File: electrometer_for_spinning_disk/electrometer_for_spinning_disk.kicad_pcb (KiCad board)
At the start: 2 copper layers, 40 x 60 mm, 22 parts, among them J1 Conn_01x01_Pin, J2 Conn_01x03_Pin, J3 Screw_Terminal_01x03, J4 PRT-14417, J5 Conn_01x01_Pin, J7 Conn_01x03_Pin, U1 LMC6082, U2 ADS1115IDGS, U3 REF3025

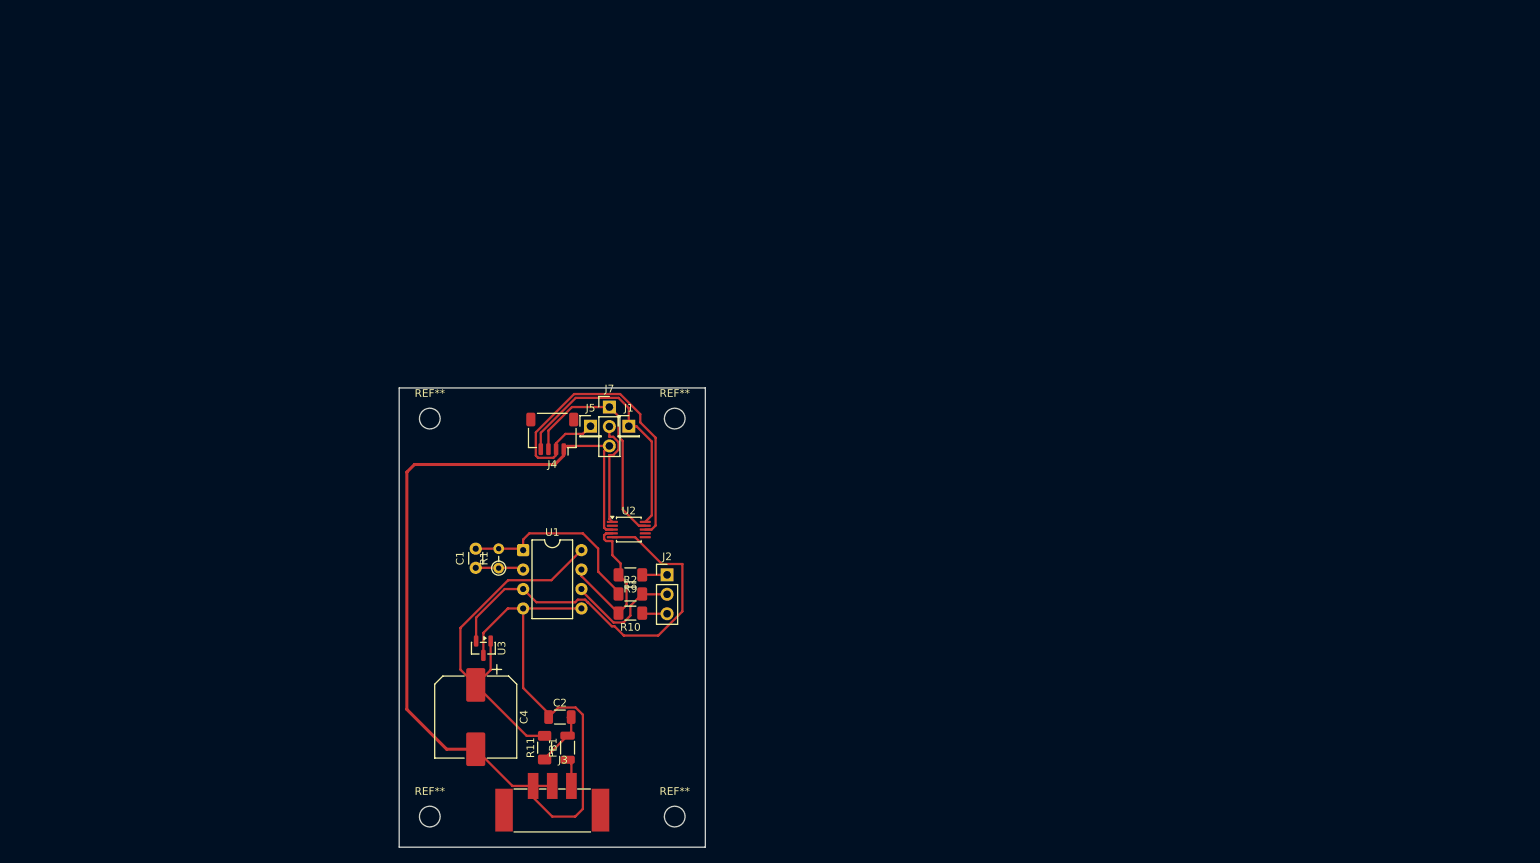
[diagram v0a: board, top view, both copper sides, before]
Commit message: perfunctory commit
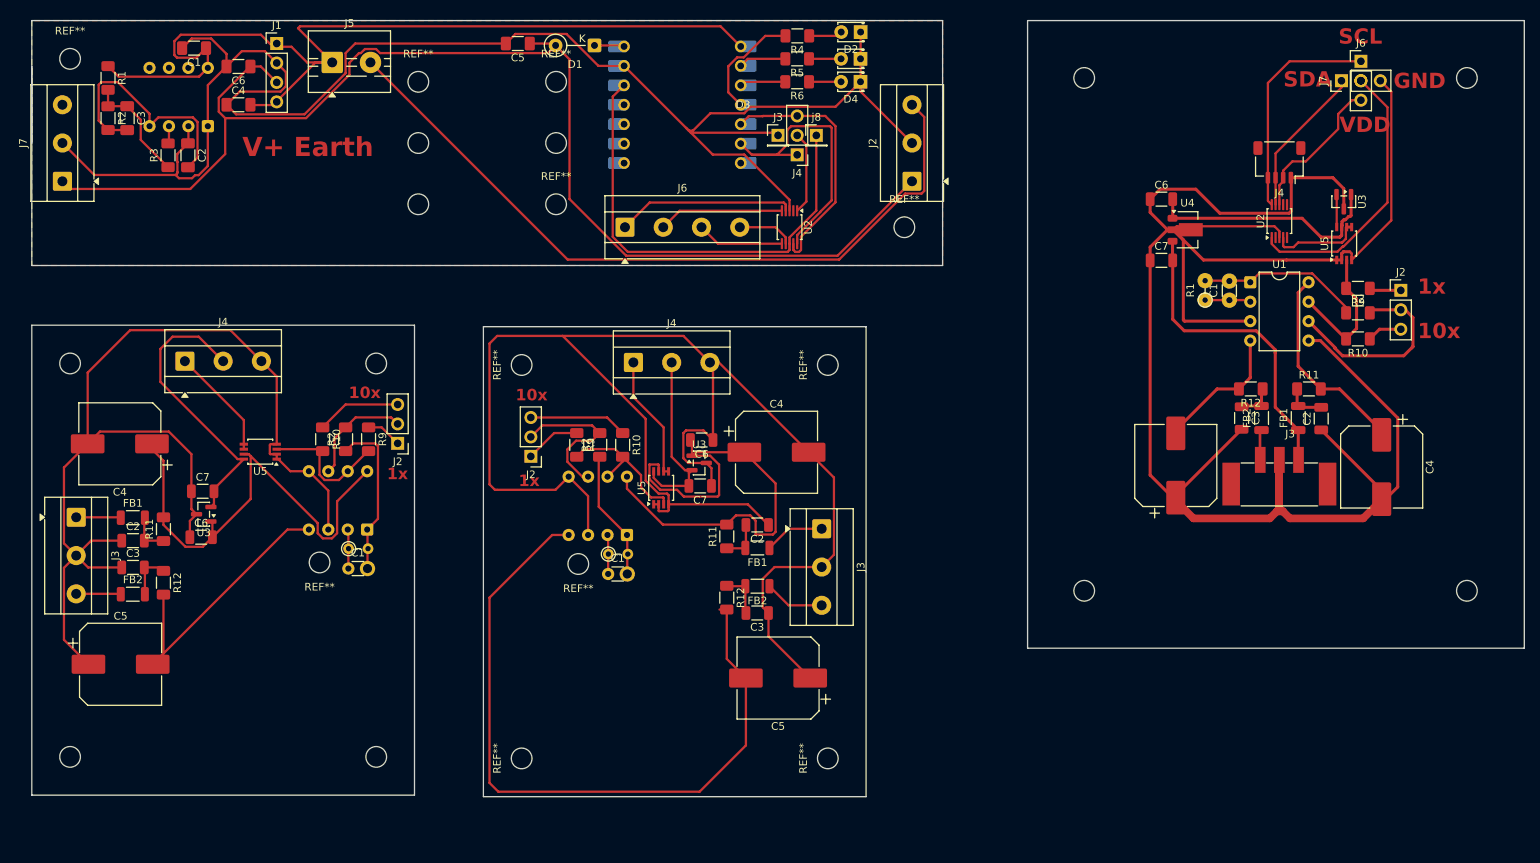
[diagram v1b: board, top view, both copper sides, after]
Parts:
- removed the C1 at (70.0, 83.5)
- removed the C2 at (81.0, 103.0)
- removed the C4 at (70.0, 103.0)
- removed the FB1 at (82.0, 107.0)
- removed the J2 at (95.0, 84.4)
- removed the J3 at (80.0, 114.1)
- removed the J4 at (80.0, 66.0)
- removed the J7 at (87.5, 62.5)
- removed the R1 at (73.0, 83.5)
- removed the R10 at (90.2, 89.4)
- removed the R11 at (79.0, 107.0)
- removed the R2 at (90.2, 86.9)
- removed the R9 at (90.2, 84.4)
- removed the REF** at (96.0, 116.0)
- removed the REF** at (96.0, 64.0)
- removed the REF** at (64.0, 64.0)
- removed the REF** at (64.0, 116.0)
- removed the U1 at (76.2, 81.2)
- removed the U2 at (90.0, 78.5)
- removed the U3 at (71.0, 94.0)
- added C1: 100p, Capacitor_THT:C_Disc_D3.0mm_W1.6mm_P2.50mm, F.Cu at (168.5, 48.5)
- added C1: 100p, Capacitor_THT:C_Disc_D3.0mm_W1.6mm_P2.50mm, F.Cu at (53.4, 83.6)
- added C1: 100p, Capacitor_THT:C_Disc_D3.0mm_W1.6mm_P2.50mm, F.Cu at (87.3, 84.3)
- added C1: 10u, Capacitor_SMD:C_1206_3216Metric_Pad1.33x1.80mm_HandSolder, F.Cu at (33.2, 15.6)
- added C2: 10u, Capacitor_SMD:C_1206_3216Metric_Pad1.33x1.80mm_HandSolder, F.Cu at (32.4, 29.6)
- added C2: 100n, Capacitor_SMD:C_1206_3216Metric, F.Cu at (106.8, 77.9)
- added C2: 100n, Capacitor_SMD:C_1206_3216Metric, F.Cu at (25.2, 80.0)
- added C2: 100n, Capacitor_SMD:C_1206_3216Metric, F.Cu at (180.5, 64.0)
- added C3: 100n, Capacitor_SMD:C_1206_3216Metric, F.Cu at (170.1, 63.9)
- added C3: 100n, Capacitor_SMD:C_1206_3216Metric, F.Cu at (25.2, 83.5)
- added C3: 100n, Capacitor_SMD:C_1206_3216Metric, F.Cu at (106.8, 89.4)
- added C3: 470n, Capacitor_SMD:C_1206_3216Metric_Pad1.33x1.80mm_HandSolder, F.Cu at (24.5, 24.8)
- added C4: C_Polarized, Capacitor_SMD:CP_Elec_10x10.5, F.Cu at (109.3, 68.4)
- added C4: 10u, Capacitor_SMD:C_1206_3216Metric_Pad1.33x1.80mm_HandSolder, F.Cu at (39.0, 23.0)
- added C4: C_Polarized, Capacitor_SMD:CP_Elec_10x10.5, F.Cu at (188.4, 70.3)
- added C4: C_Polarized, Capacitor_SMD:CP_Elec_10x10.5, F.Cu at (23.5, 67.3)
- added C5: C_Polarized, Capacitor_SMD:CP_Elec_10x10.5, F.Cu at (161.5, 70.1)
- added C5: 10u, Capacitor_SMD:C_1206_3216Metric_Pad1.33x1.80mm_HandSolder, F.Cu at (75.5, 15.0)
- added C5: C_Polarized, Capacitor_SMD:CP_Elec_10x10.5, F.Cu at (23.6, 96.1)
- added C5: C_Polarized, Capacitor_SMD:CP_Elec_10x10.5, F.Cu at (109.5, 97.9)
- added C6: 10u, Capacitor_SMD:C_1206_3216Metric_Pad1.33x1.80mm_HandSolder, F.Cu at (39.0, 18.0)
- added C6: 100n, Capacitor_SMD:C_1206_3216Metric, F.Cu at (159.6, 35.3)
- added C6: 100n, Capacitor_SMD:C_1206_3216Metric, F.Cu at (34.1, 79.5)
- added C6: 100n, Capacitor_SMD:C_1206_3216Metric, F.Cu at (99.5, 66.8)
- added C7: 100n, Capacitor_SMD:C_1206_3216Metric, F.Cu at (34.3, 73.5)
- added C7: 100n, Capacitor_SMD:C_1206_3216Metric, F.Cu at (99.3, 72.8)
- added C7: 100n, Capacitor_SMD:C_1206_3216Metric, F.Cu at (159.6, 43.3)
- added D1: D_Schottky, Diode_THT:D_A-405_P5.08mm_Vertical_CathodeUp, F.Cu at (85.5, 15.2)
- added D2: LED, LED_THT:LED_D1.8mm_W3.3mm_H2.4mm, F.Cu at (120.3, 13.5)
- added D3: LED, LED_THT:LED_D1.8mm_W3.3mm_H2.4mm, F.Cu at (120.3, 17.0)
- added D4: LED, LED_THT:LED_D1.8mm_W3.3mm_H2.4mm, F.Cu at (120.3, 20.0)
- added FB1: FerriteBead, Inductor_SMD:L_1206_3216Metric, F.Cu at (177.5, 63.9)
- added FB1: FerriteBead, Inductor_SMD:L_1206_3216Metric, F.Cu at (25.2, 77.0)
- added FB1: FerriteBead, Inductor_SMD:L_1206_3216Metric, F.Cu at (106.8, 80.9)
- added FB2: FerriteBead, Inductor_SMD:L_1206_3216Metric, F.Cu at (106.8, 85.9)
- added FB2: FerriteBead, Inductor_SMD:L_1206_3216Metric, F.Cu at (172.7, 63.9)
- added FB2: FerriteBead, Inductor_SMD:L_1206_3216Metric, F.Cu at (25.2, 87.0)
- added J2: Electro Power1, TerminalBlock_MetzConnect:TerminalBlock_MetzConnect_Type055_RT01503HDWU_1x03_P5.00mm_Horizontal, F.Cu at (127.0, 33.0)
- added J2: Conn_01x03_Pin, Connector_PinHeader_2.54mm:PinHeader_1x03_P2.54mm_Vertical, F.Cu at (77.2, 68.9)
- added J2: Conn_01x03_Pin, Connector_PinHeader_2.54mm:PinHeader_1x03_P2.54mm_Vertical, F.Cu at (59.8, 67.2)
- added J2: Conn_01x03_Pin, Connector_PinHeader_2.54mm:PinHeader_1x03_P2.54mm_Vertical, F.Cu at (190.9, 47.3)
- added J3: Screw_Terminal_01x03, TerminalBlock_Phoenix:TerminalBlock_Phoenix_PTSM-0,5-3-2,5-V-SMD_1x03-1MP_P2.50mm_Vertical, F.Cu at (175.0, 71.5)
- added J3: Conn_01x01_Pin, Connector_PinHeader_2.54mm:PinHeader_1x01_P2.54mm_Vertical, F.Cu at (109.5, 27.0)
- added J3: Screw_Terminal_01x03, TerminalBlock_MetzConnect:TerminalBlock_MetzConnect_Type055_RT01503HDWU_1x03_P5.00mm_Horizontal, F.Cu at (115.2, 78.4)
- added J3: Screw_Terminal_01x03, TerminalBlock_MetzConnect:TerminalBlock_MetzConnect_Type055_RT01503HDWU_1x03_P5.00mm_Horizontal, F.Cu at (17.8, 76.9)
- added J4: PRT-14417, Connector_JST:JST_SH_SM04B-SRSS-TB_1x04-1MP_P1.00mm_Horizontal, F.Cu at (175.0, 30.5)
- added J4: Screw_Terminal_01x03, TerminalBlock_MetzConnect:TerminalBlock_MetzConnect_Type055_RT01503HDWU_1x03_P5.00mm_Horizontal, F.Cu at (90.6, 56.7)
- added J4: Conn_01x03_Pin, Connector_PinHeader_2.54mm:PinHeader_1x03_P2.54mm_Vertical, F.Cu at (112.0, 29.5)
- added J4: Screw_Terminal_01x03, TerminalBlock_MetzConnect:TerminalBlock_MetzConnect_Type055_RT01503HDWU_1x03_P5.00mm_Horizontal, F.Cu at (32.0, 56.5)
- added J6: Screw_Terminal_01x04, TerminalBlock_MetzConnect:TerminalBlock_MetzConnect_Type055_RT01504HDWU_1x04_P5.00mm_Horizontal, F.Cu at (89.5, 39.0)
- added J6: Conn_01x03_Pin, Connector_PinHeader_2.54mm:PinHeader_1x03_P2.54mm_Vertical, F.Cu at (185.6, 17.3)
- added J7: Conn_01x03_Pin, Connector_PinHeader_2.54mm:PinHeader_1x03_P2.54mm_Vertical, F.Cu at (183.1, 19.9)
- added J7: Electro Power2, TerminalBlock_MetzConnect:TerminalBlock_MetzConnect_Type055_RT01503HDWU_1x03_P5.00mm_Horizontal, F.Cu at (16.0, 33.0)
- added R1: 5G, Resistor_THT:R_Axial_DIN0204_L3.6mm_D1.6mm_P2.54mm_Vertical, F.Cu at (165.3, 48.5)
- added R1: 5G, Resistor_THT:R_Axial_DIN0204_L3.6mm_D1.6mm_P2.54mm_Vertical, F.Cu at (53.4, 81.0)
- added R1: 5G, Resistor_THT:R_Axial_DIN0204_L3.6mm_D1.6mm_P2.54mm_Vertical, F.Cu at (87.3, 81.7)
- added R1: 20k, Resistor_SMD:R_1206_3216Metric_Pad1.30x1.75mm_HandSolder, F.Cu at (22.0, 19.5)
- added R10: 10k, Resistor_SMD:R_1206_3216Metric_Pad1.30x1.75mm_HandSolder, F.Cu at (50.0, 66.7)
- added R10: 10k, Resistor_SMD:R_1206_3216Metric_Pad1.30x1.75mm_HandSolder, F.Cu at (185.3, 53.6)
- added R10: 10k, Resistor_SMD:R_1206_3216Metric_Pad1.30x1.75mm_HandSolder, F.Cu at (89.2, 67.4)
- added R11: 1k, Resistor_SMD:R_1206_3216Metric_Pad1.30x1.75mm_HandSolder, F.Cu at (29.2, 78.5)
- added R11: 10, Resistor_SMD:R_1206_3216Metric_Pad1.30x1.75mm_HandSolder, F.Cu at (178.9, 60.1)
- added R11: 1k, Resistor_SMD:R_1206_3216Metric_Pad1.30x1.75mm_HandSolder, F.Cu at (102.8, 79.4)
- added R12: 10, Resistor_SMD:R_1206_3216Metric_Pad1.30x1.75mm_HandSolder, F.Cu at (171.3, 60.1)
- added R12: 1k, Resistor_SMD:R_1206_3216Metric_Pad1.30x1.75mm_HandSolder, F.Cu at (29.2, 85.5)
- added R12: 1k, Resistor_SMD:R_1206_3216Metric_Pad1.30x1.75mm_HandSolder, F.Cu at (102.8, 87.4)
- added R2: 10k, Resistor_SMD:R_1206_3216Metric_Pad1.30x1.75mm_HandSolder, F.Cu at (22.0, 24.8)
- added R2: 1k, Resistor_SMD:R_1206_3216Metric_Pad1.30x1.75mm_HandSolder, F.Cu at (53.0, 66.7)
- added R2: 1k, Resistor_SMD:R_1206_3216Metric_Pad1.30x1.75mm_HandSolder, F.Cu at (185.3, 50.2)
- added R2: 1k, Resistor_SMD:R_1206_3216Metric_Pad1.30x1.75mm_HandSolder, F.Cu at (86.2, 67.4)
- added R3: 1k, Resistor_SMD:R_1206_3216Metric_Pad1.30x1.75mm_HandSolder, F.Cu at (29.8, 29.6)
- added R4: 1k, Resistor_SMD:R_1206_3216Metric_Pad1.30x1.75mm_HandSolder, F.Cu at (112.0, 14.0)
- added R5: 1k, Resistor_SMD:R_1206_3216Metric_Pad1.30x1.75mm_HandSolder, F.Cu at (112.0, 17.0)
- added R6: 1k, Resistor_SMD:R_1206_3216Metric_Pad1.30x1.75mm_HandSolder, F.Cu at (112.0, 20.0)
- added R9: 1k, Resistor_SMD:R_1206_3216Metric_Pad1.30x1.75mm_HandSolder, F.Cu at (185.3, 47.0)
- added R9: 1k, Resistor_SMD:R_1206_3216Metric_Pad1.30x1.75mm_HandSolder, F.Cu at (56.0, 66.7)
- added R9: 1k, Resistor_SMD:R_1206_3216Metric_Pad1.30x1.75mm_HandSolder, F.Cu at (83.2, 67.4)
- added REF**: MountingHole_2.7mm_M2.5_ISO14580, MountingHole:MountingHole_2.7mm_M2.5_ISO14580, F.Cu at (83.4, 83.0)
- added REF**: MountingHole_2.7mm_M2.5, MountingHole:MountingHole_2.7mm_M2.5, F.Cu at (80.5, 36.0)
- added REF**: MountingHole_2.7mm, MountingHole:MountingHole_2.7mm, F.Cu at (199.5, 19.5)
- added REF**: MountingHole_2.7mm_M2.5_ISO14580, MountingHole:MountingHole_2.7mm_M2.5_ISO14580, F.Cu at (76.0, 108.4)
- added REF**: MountingHole_2.7mm_M2.5, MountingHole:MountingHole_2.7mm_M2.5, F.Cu at (62.5, 20.0)
- added REF**: MountingHole_2.7mm, MountingHole:MountingHole_2.7mm, F.Cu at (149.5, 86.5)
- added REF**: MountingHole_2.7mm_M2.5_ISO14580, MountingHole:MountingHole_2.7mm_M2.5_ISO14580, F.Cu at (116.0, 108.4)
- added REF**: MountingHole_2.7mm_M2.5, MountingHole:MountingHole_2.7mm_M2.5, F.Cu at (62.5, 28.0)
- added REF**: MountingHole_2.7mm_M2.5_ISO14580, MountingHole:MountingHole_2.7mm_M2.5_ISO14580, F.Cu at (57.0, 108.2)
- added REF**: MountingHole_2.7mm_M2.5_ISO14580, MountingHole:MountingHole_2.7mm_M2.5_ISO14580, F.Cu at (116.0, 57.0)
- added REF**: MountingHole_2.7mm_M2.5, MountingHole:MountingHole_2.7mm_M2.5, F.Cu at (17.0, 17.0)
- added REF**: MountingHole_2.7mm, MountingHole:MountingHole_2.7mm, F.Cu at (199.5, 86.5)
- added REF**: MountingHole_2.7mm_M2.5, MountingHole:MountingHole_2.7mm_M2.5, F.Cu at (62.5, 36.0)
- added REF**: MountingHole_2.7mm_M2.5_ISO14580, MountingHole:MountingHole_2.7mm_M2.5_ISO14580, F.Cu at (17.0, 108.2)
- added REF**: MountingHole_2.7mm_M2.5_ISO14580, MountingHole:MountingHole_2.7mm_M2.5_ISO14580, F.Cu at (17.0, 56.8)
- added REF**: MountingHole_2.7mm_M2.5, MountingHole:MountingHole_2.7mm_M2.5, F.Cu at (80.5, 20.0)
- added REF**: MountingHole_2.7mm_M2.5_ISO14580, MountingHole:MountingHole_2.7mm_M2.5_ISO14580, F.Cu at (57.0, 56.8)
- added REF**: MountingHole_2.7mm_M2.5_ISO14580, MountingHole:MountingHole_2.7mm_M2.5_ISO14580, F.Cu at (49.6, 82.8)
- added REF**: MountingHole_2.7mm, MountingHole:MountingHole_2.7mm, F.Cu at (149.5, 19.5)
- added REF**: MountingHole_2.7mm_M2.5, MountingHole:MountingHole_2.7mm_M2.5, F.Cu at (80.5, 28.0)
- added REF**: MountingHole_2.7mm_M2.5_ISO14580, MountingHole:MountingHole_2.7mm_M2.5_ISO14580, F.Cu at (76.0, 57.0)
- added REF**: MountingHole_2.7mm_M2.5, MountingHole:MountingHole_2.7mm_M2.5, F.Cu at (126.0, 39.0)
- added U1: LMC6082, Package_DIP:DIP-8_W7.62mm, F.Cu at (171.2, 46.2)
- added U1: LMC6082, Package_DIP:DIP-8_W7.62mm, B.Cu at (55.8, 78.5)
- added U1: LMC6082, Package_DIP:DIP-8_W7.62mm, B.Cu at (89.8, 79.2)
- added U1: LM358, Package_DIP:DIP-8_W7.62mm, B.Cu at (35.0, 25.8)
- added U2: ADS1115IDGS, Package_SO:TSSOP-10_3x3mm_P0.5mm, F.Cu at (111.0, 39.0)
- added U2: ADS1115IDGS, Package_SO:TSSOP-10_3x3mm_P0.5mm, F.Cu at (175.0, 38.2)
- added U3: REF3025, Package_TO_SOT_SMD:SOT-23, F.Cu at (183.4, 35.7)
- added U3: REF3025, Package_TO_SOT_SMD:SOT-23, F.Cu at (99.2, 69.8)
- added U3: REF3025, Package_TO_SOT_SMD:SOT-23, F.Cu at (34.5, 76.5)
- added U3: XIAO ESP32C3, xiao:XIAO-ESP32-C6-DIP, B.Cu at (97.0, 23.0)
- added U4: 5V LDO, Package_TO_SOT_SMD:SOT-89-3, F.Cu at (163.0, 39.3)
- added U5: INA159AIDGKR, Package_SO:TSSOP-8_3x3mm_P0.65mm, F.Cu at (183.5, 41.1)
- added U5: INA159AIDGKR, Package_SO:TSSOP-8_3x3mm_P0.65mm, F.Cu at (94.2, 73.0)
- added U5: INA159AIDGKR, Package_SO:TSSOP-8_3x3mm_P0.65mm, F.Cu at (41.9, 68.3)
- added j8: Conn_01x01_Pin, Connector_PinHeader_2.54mm:PinHeader_1x01_P2.54mm_Vertical, F.Cu at (114.5, 27.0)
- J1: value Conn_01x01_Pin -> TPS61023; footprint Connector_PinHeader_2.54mm:PinHeader_1x01_P2.54mm_Vertical -> Connector_PinHeader_2.54mm:PinHeader_1x04_P2.54mm_Vertical
- J5: value Conn_01x01_Pin -> Inductive Charging; footprint Connector_PinHeader_2.54mm:PinHeader_1x01_P2.54mm_Vertical -> TerminalBlock:TerminalBlock_MaiXu_MX126-5.0-02P_1x02_P5.00mm
- moved J1 67.9 mm to (44.0, 15.0)
- moved J5 58.3 mm to (51.2, 17.5)
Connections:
- J1 pad 1: /Yellow -> +5V
- J5 pad 1: +3.3V -> +5V
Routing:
- net GND: track 154.4 -> 601.0 mm
- net GNDREF: track 0.00 -> 217.0 mm
- net +5VP: track 0.00 -> 166.1 mm
- net +5V: track 3.63 -> 156.0 mm
- net -VDC: track 0.00 -> 131.6 mm
- net Earth: track 0.00 -> 131.1 mm
- net +VDC: track 0.00 -> 130.5 mm
- net /VDD: track 0.00 -> 60.9 mm
- net /Output: track 0.00 -> 49.6 mm
- net VDD: track 46.6 -> 0.00 mm
- net Net-(J2-Pin_2): track 15.4 -> 61.0 mm
- net V+: track 0.00 -> 40.9 mm
- net /SCL: track 0.00 -> 38.2 mm
- net Net-(C1-Pad2): track 25.5 -> 59.8 mm
- net /SDA: track 0.00 -> 33.5 mm
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- added copper zone on F.Cu, net Earth
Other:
- board size 40 x 60 mm -> 195 x 101.4 mm
- board text added: "10x"
- board text added: "1x"
- board text added: "GND"
- board text added: "SCL"
- board text added: "SDA"
- board text added: "V+ Earth"
- board text added: "VDD"

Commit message: lots of new stuff
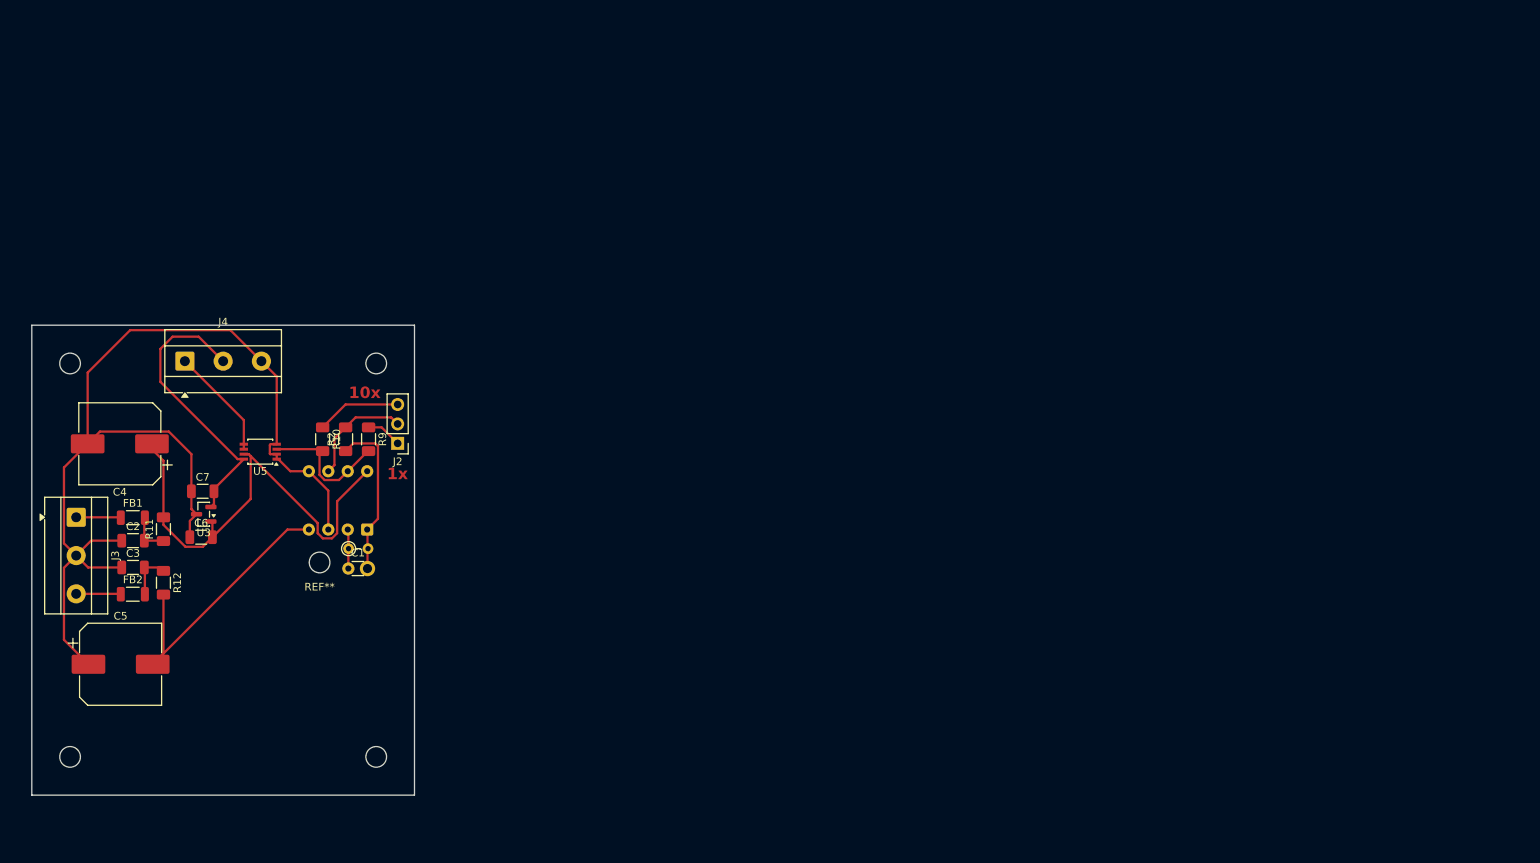
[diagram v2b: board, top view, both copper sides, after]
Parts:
- removed the C1 at (168.5, 48.5)
- removed the C1 at (87.3, 84.3)
- removed the C1 at (33.2, 15.6)
- removed the C2 at (32.4, 29.6)
- removed the C2 at (106.8, 77.9)
- removed the C2 at (180.5, 64.0)
- removed the C3 at (170.1, 63.9)
- removed the C3 at (106.8, 89.4)
- removed the C3 at (24.5, 24.8)
- removed the C4 at (109.3, 68.4)
- removed the C4 at (39.0, 23.0)
- removed the C4 at (188.4, 70.3)
- removed the C5 at (161.5, 70.1)
- removed the C5 at (75.5, 15.0)
- removed the C5 at (109.5, 97.9)
- removed the C6 at (39.0, 18.0)
- removed the C6 at (159.6, 35.3)
- removed the C6 at (99.5, 66.8)
- removed the C7 at (99.3, 72.8)
- removed the C7 at (159.6, 43.3)
- removed D1: D_Schottky, Diode_THT:D_A-405_P5.08mm_Vertical_CathodeUp
- removed D2, D3, D4: LED, LED_THT:LED_D1.8mm_W3.3mm_H2.4mm
- removed the FB1 at (177.5, 63.9)
- removed the FB1 at (106.8, 80.9)
- removed the FB2 at (106.8, 85.9)
- removed the FB2 at (172.7, 63.9)
- removed J1: TPS61023, Connector_PinHeader_2.54mm:PinHeader_1x04_P2.54mm_Vertical
- removed the J2 at (127.0, 33.0)
- removed the J2 at (77.2, 68.9)
- removed the J2 at (190.9, 47.3)
- removed the J3 at (175.0, 71.5)
- removed the J3 at (109.5, 27.0)
- removed the J3 at (115.2, 78.4)
- removed the J4 at (175.0, 30.5)
- removed the J4 at (90.6, 56.7)
- removed the J4 at (112.0, 29.5)
- removed J5: Inductive Charging, TerminalBlock:TerminalBlock_MaiXu_MX126-5.0-02P_1x02_P5.00mm
- removed J6: Screw_Terminal_01x04, TerminalBlock_MetzConnect:TerminalBlock_MetzConnect_Type055_RT01504HDWU_1x04_P5.00mm_Horizontal
- removed J6, J7: Conn_01x03_Pin, Connector_PinHeader_2.54mm:PinHeader_1x03_P2.54mm_Vertical
- removed J7: Electro Power2, TerminalBlock_MetzConnect:TerminalBlock_MetzConnect_Type055_RT01503HDWU_1x03_P5.00mm_Horizontal
- removed the R1 at (165.3, 48.5)
- removed the R1 at (87.3, 81.7)
- removed the R1 at (22.0, 19.5)
- removed the R10 at (185.3, 53.6)
- removed the R10 at (89.2, 67.4)
- removed the R11 at (178.9, 60.1)
- removed the R11 at (102.8, 79.4)
- removed the R12 at (171.3, 60.1)
- removed the R12 at (102.8, 87.4)
- removed the R2 at (22.0, 24.8)
- removed the R2 at (185.3, 50.2)
- removed the R2 at (86.2, 67.4)
- removed R3, R4, R5, R6: 1k, Resistor_SMD:R_1206_3216Metric_Pad1.30x1.75mm_HandSolder
- removed the R9 at (185.3, 47.0)
- removed the R9 at (83.2, 67.4)
- removed the REF** at (83.4, 83.0)
- removed the REF** at (80.5, 36.0)
- removed the REF** at (199.5, 19.5)
- removed the REF** at (76.0, 108.4)
- removed the REF** at (62.5, 20.0)
- removed the REF** at (149.5, 86.5)
- removed the REF** at (116.0, 108.4)
- removed the REF** at (62.5, 28.0)
- removed the REF** at (116.0, 57.0)
- removed the REF** at (17.0, 17.0)
- removed the REF** at (199.5, 86.5)
- removed the REF** at (62.5, 36.0)
- removed the REF** at (80.5, 20.0)
- removed the REF** at (149.5, 19.5)
- removed the REF** at (80.5, 28.0)
- removed the REF** at (76.0, 57.0)
- removed the REF** at (126.0, 39.0)
- removed the U1 at (171.2, 46.2)
- removed the U1 at (89.8, 79.2)
- removed the U1 at (35.0, 25.8)
- removed U2 (x2): ADS1115IDGS, Package_SO:TSSOP-10_3x3mm_P0.5mm
- removed the U3 at (183.4, 35.7)
- removed the U3 at (99.2, 69.8)
- removed the U3 at (97.0, 23.0)
- removed U4: 5V LDO, Package_TO_SOT_SMD:SOT-89-3
- removed the U5 at (183.5, 41.1)
- removed the U5 at (94.2, 73.0)
- removed j8: Conn_01x01_Pin, Connector_PinHeader_2.54mm:PinHeader_1x01_P2.54mm_Vertical
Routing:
- net GND: track 601.0 -> 137.9 mm
- net GNDREF: track 217.0 -> 0.00 mm
- net +5VP: track 166.1 -> 0.00 mm
- net +5V: track 156.0 -> 0.00 mm
- net Earth: track 131.1 -> 0.00 mm
- net -VDC: track 131.6 -> 37.4 mm
- net +VDC: track 130.5 -> 61.5 mm
- net /VDD: track 60.9 -> 0.00 mm
- net /ADDR: track 47.2 -> 0.00 mm
- net Net-(J2-Pin_2): track 61.0 -> 14.4 mm
- net V+: track 40.9 -> 0.00 mm
- net Net-(C1-Pad2): track 59.8 -> 21.4 mm
- net /SCL: track 38.2 -> 0.00 mm
- net /Output: track 49.6 -> 14.7 mm
- net /SDA: track 33.5 -> 0.00 mm
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- removed copper zone on F.Cu, net Earth
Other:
- board size 195 x 101.4 mm -> 50 x 61.4 mm
- board text removed: "GND"
- board text removed: "SCL"
- board text removed: "SDA"
- board text removed: "V+ Earth"
- board text removed: "VDD"
